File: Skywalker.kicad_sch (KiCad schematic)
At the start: 55 parts

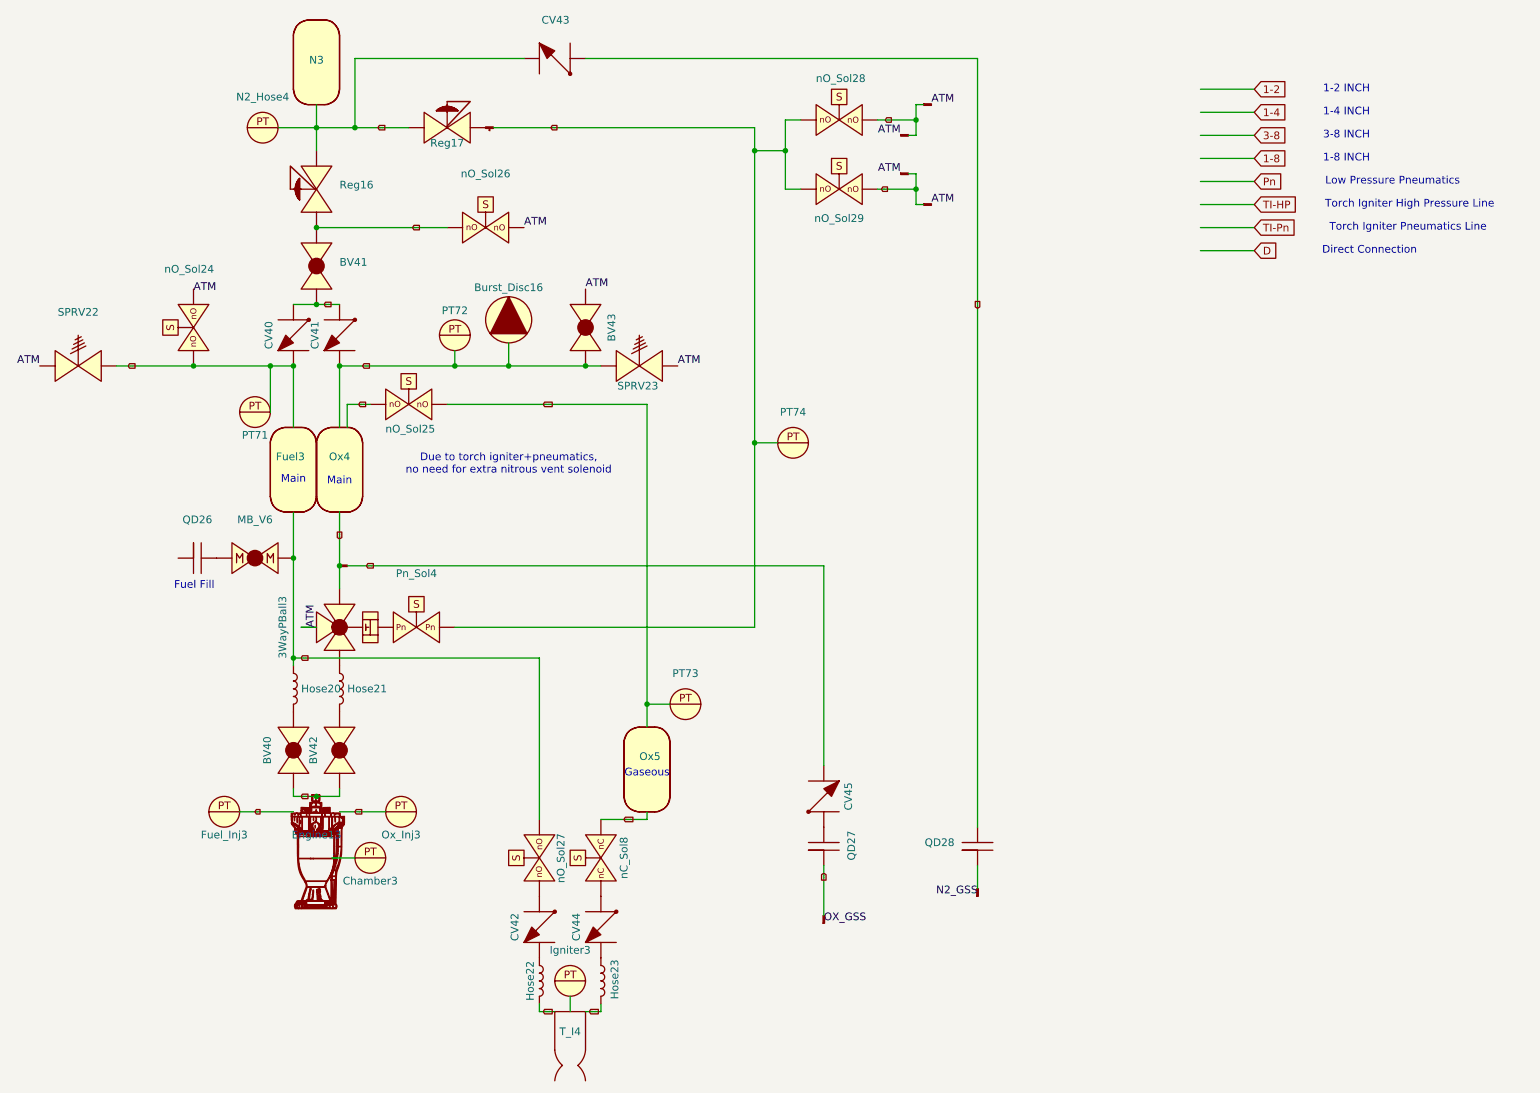
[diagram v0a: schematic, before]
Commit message: j0
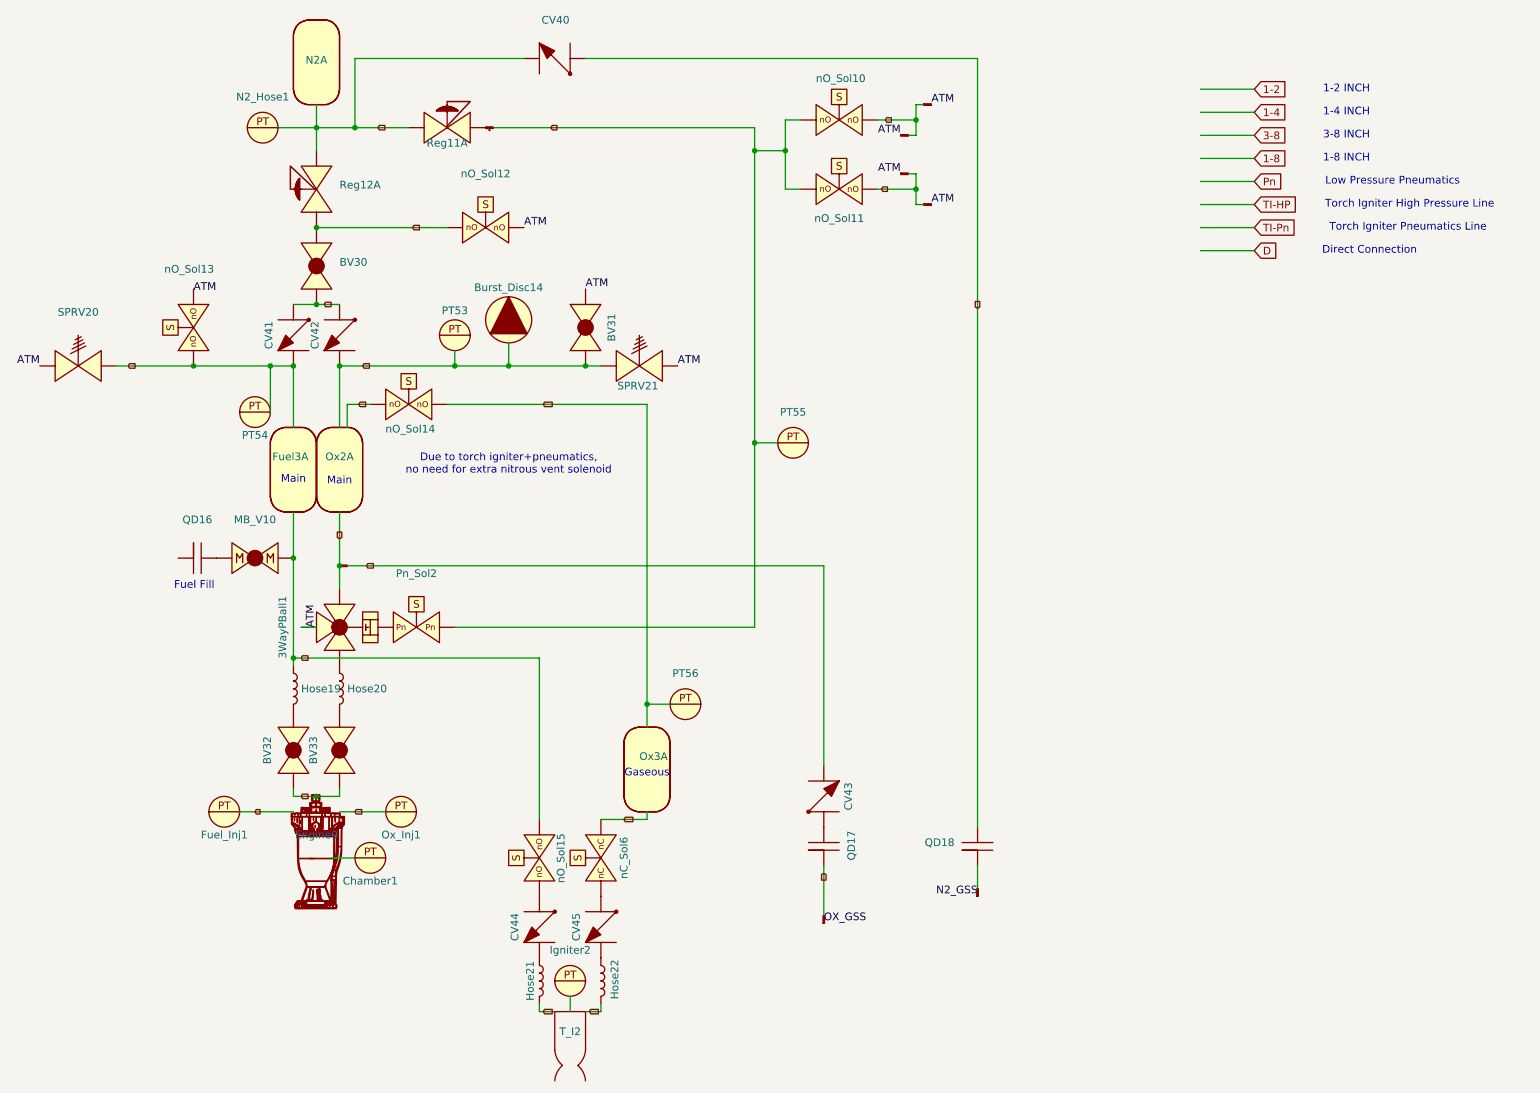
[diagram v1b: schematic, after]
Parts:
- renumbered 3WayPBall3 to 3WayPBall1, BV41 to BV30, BV43 to BV31, BV40 to BV32, BV42 to BV33, Burst_Disc16 to Burst_Disc14, CV43 to CV40, CV40 to CV41, CV41 to CV42, CV45 to CV43, CV42 to CV44, CV44 to CV45, Chamber3 to Chamber1, Engine13 to Engine9, Fuel_Inj3 to Fuel_Inj1, Hose20 to Hose19, Hose21 to Hose20, Hose22 to Hose21, Hose23 to Hose22, Igniter3 to Igniter2, MB_V6 to MB_V10, N3 to N2, N2_Hose4 to N2_Hose1, Ox4 to Ox2, Ox5 to Ox3, Ox_Inj3 to Ox_Inj1, PT72 to PT53, PT71 to PT54, PT74 to PT55, PT73 to PT56, Pn_Sol4 to Pn_Sol2, QD26 to QD16, QD27 to QD17, QD28 to QD18, Reg17 to Reg11, Reg16 to Reg12, SPRV22 to SPRV20, SPRV23 to SPRV21, Stop2 to Stop1, T_I4 to T_I2, U41 to U40, U39 to U41, U40 to U42, U42 to U43, U37 to U44, U43 to U45, U38 to U46, nC_Sol8 to nC_Sol6, nO_Sol28 to nO_Sol10, nO_Sol29 to nO_Sol11, nO_Sol26 to nO_Sol12, nO_Sol24 to nO_Sol13, nO_Sol25 to nO_Sol14, nO_Sol27 to nO_Sol15
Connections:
- net at CV45.: now also Hose22.1; no longer nC_Sol6.
- net at QD16.: now also MB_V10.
- new net: CV45., nC_Sol6.
- new net: Reg11., Stop1.
- new net: 3WayPBall1., Pn_Sol2.
- new net: CV43., QD17.
- new net: QD18., U45.

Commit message: more silwood stuff
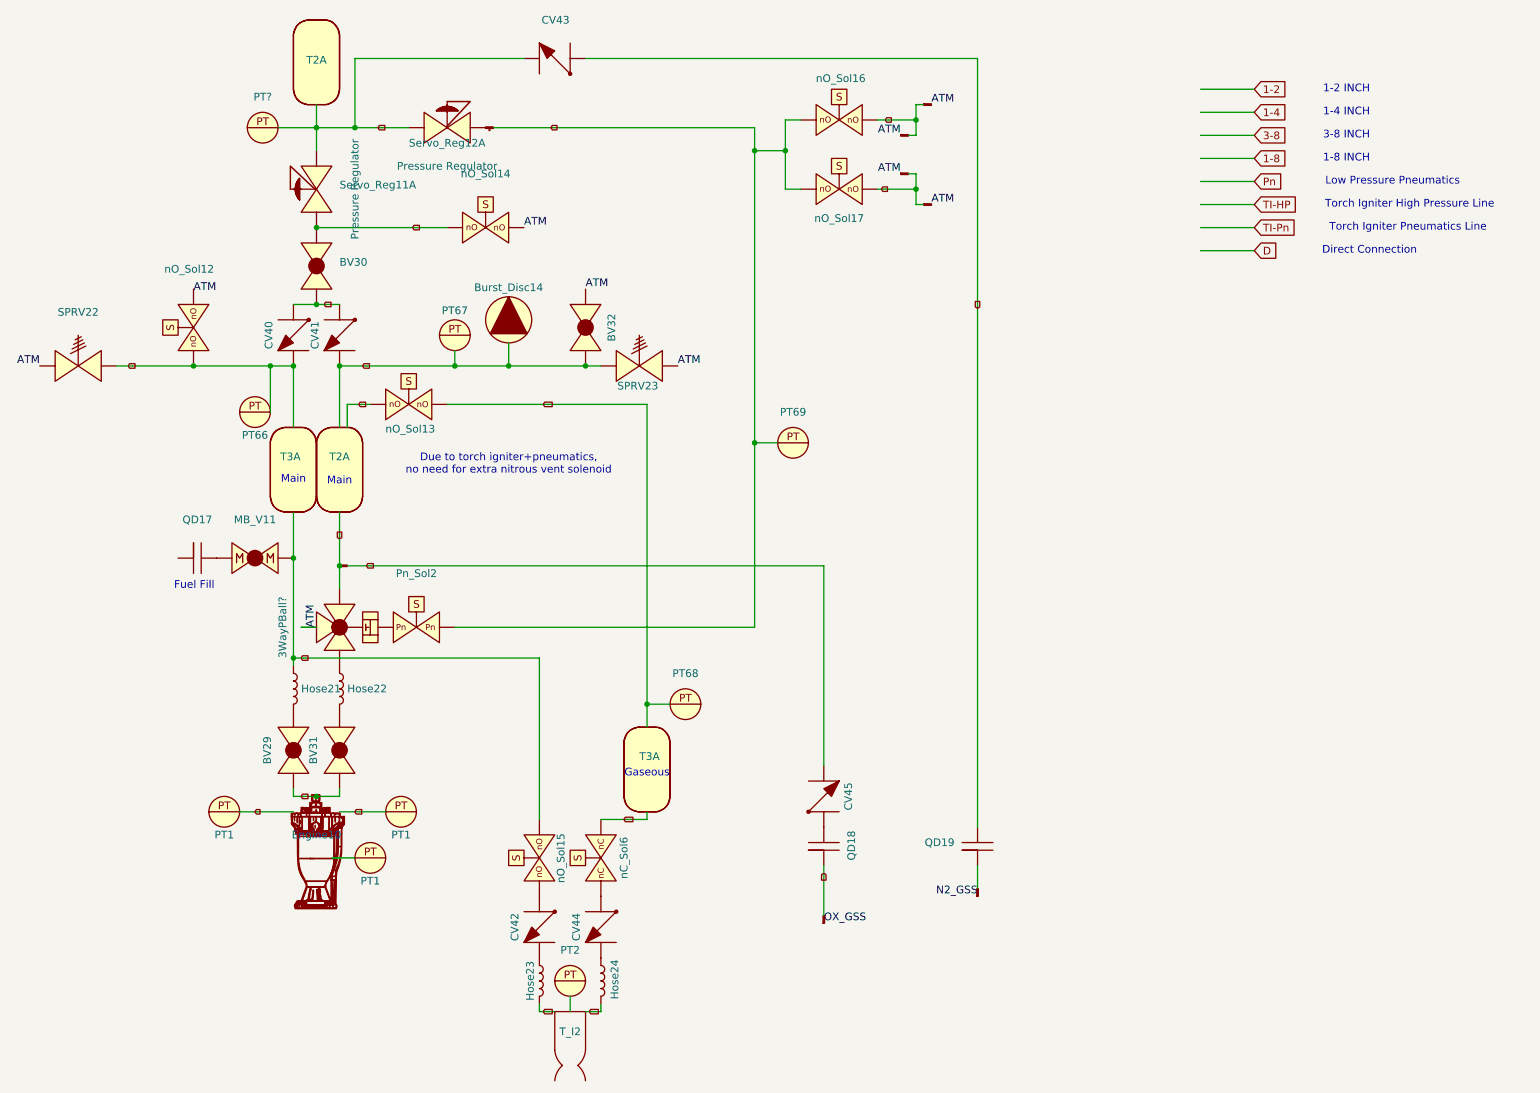
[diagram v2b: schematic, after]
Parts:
- renumbered 3WayPBall1 to 3WayPBall?, BV32 to BV29, BV33 to BV31, BV31 to BV32, CV41 to CV40, CV42 to CV41, CV44 to CV42, CV40 to CV43, CV45 to CV44, CV43 to CV45, Engine9 to Engine10, Hose19 to Hose21, Hose20 to Hose22, Hose21 to Hose23, Hose22 to Hose24, MB_V10 to MB_V11, Chamber1 to PT1, Fuel_Inj1 to PT1, Ox_Inj1 to PT1, Igniter2 to PT2, PT54 to PT66, PT53 to PT67, PT56 to PT68, PT55 to PT69, N2_Hose1 to PT?, QD16 to QD17, QD17 to QD18, QD18 to QD19, SPRV20 to SPRV22, SPRV21 to SPRV23, Reg12 to Servo_Reg11, Reg11 to Servo_Reg12, Ox2 to T2, N2 to T2, Fuel3 to T3, Ox3 to T3, U44 to U55, U46 to U56, U41 to U57, U42 to U58, U40 to U59, U43 to U60, U45 to U61, nO_Sol13 to nO_Sol12, nO_Sol14 to nO_Sol13, nO_Sol12 to nO_Sol14, nO_Sol10 to nO_Sol16, nO_Sol11 to nO_Sol17
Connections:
- net at CV44.: now also Hose24.1; no longer nC_Sol6.
- net at QD17.: now also MB_V11.
- new net: CV44., nC_Sol6.
- new net: Servo_Reg12., Stop1.
- new net: 3WayPBall?., Pn_Sol2.
- new net: CV45., QD18.
- new net: QD19., U61.

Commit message: Formatiing
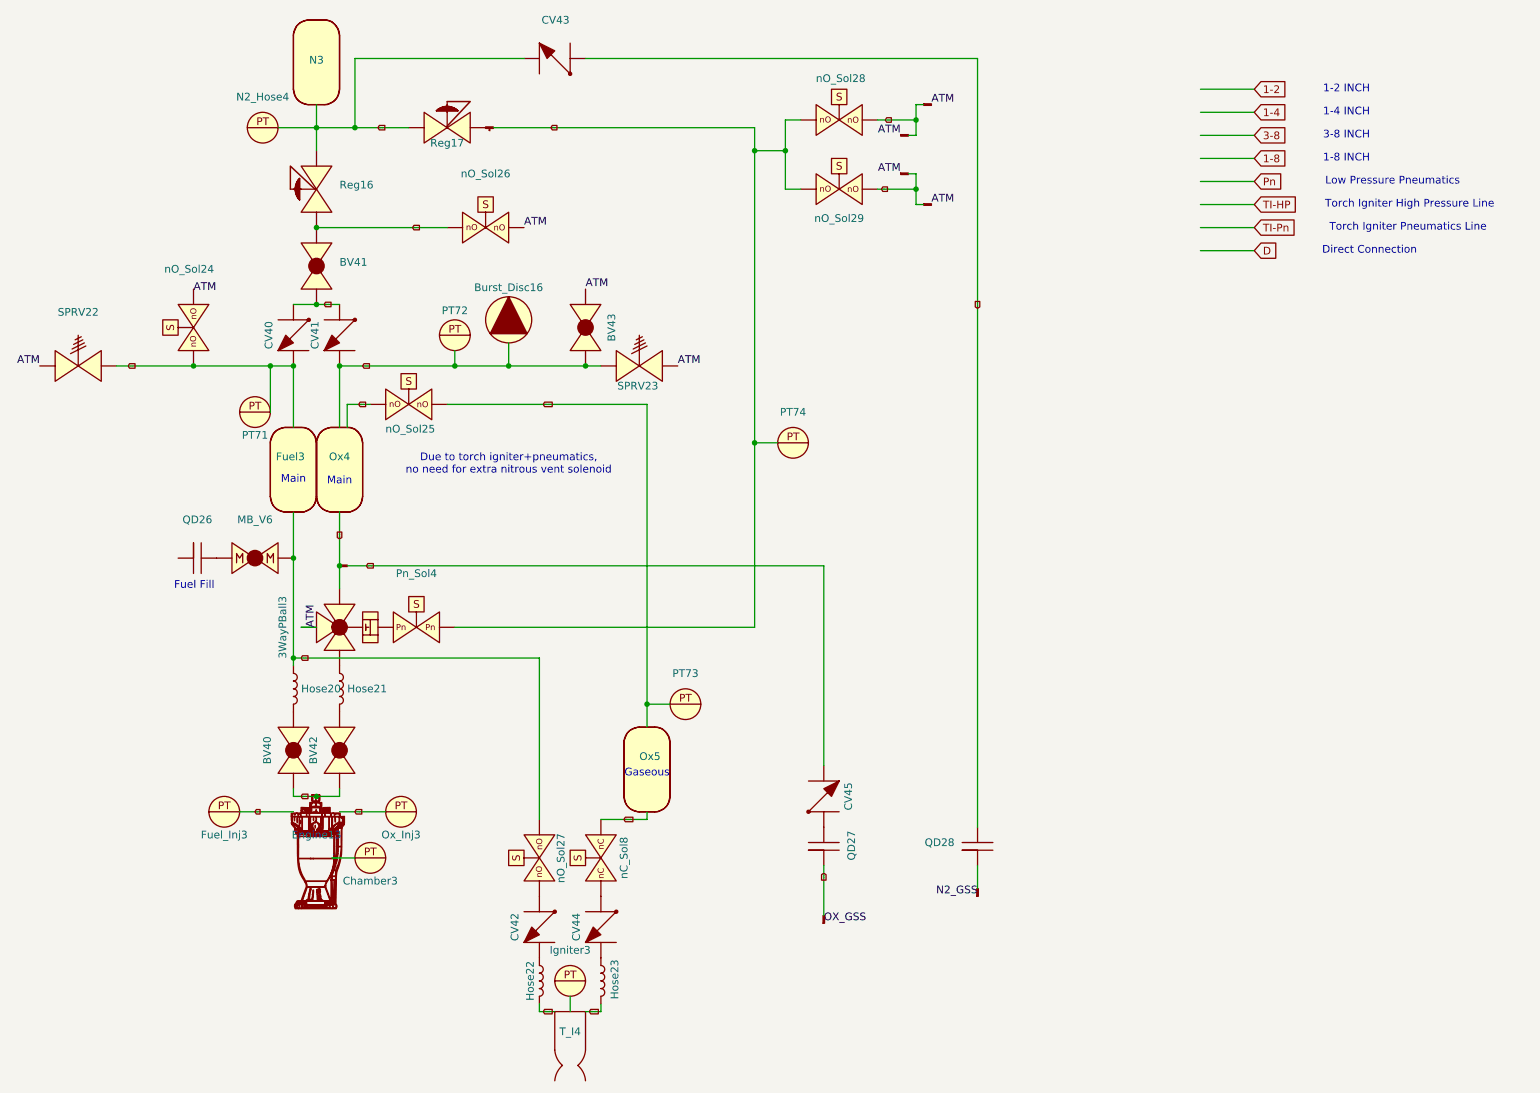
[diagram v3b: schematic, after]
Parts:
- gave numbers to parts that had none: 2
- renumbered BV29 to BV40, BV30 to BV41, BV31 to BV42, BV32 to BV43, Burst_Disc14 to Burst_Disc16, PT1 to Chamber3, Engine10 to Engine13, T3 to Fuel3, PT1 to Fuel_Inj3, Hose21 to Hose20, Hose22 to Hose21, Hose23 to Hose22, Hose24 to Hose23, PT2 to Igniter3, MB_V11 to MB_V6, T2 to N3, T2 to Ox4, T3 to Ox5, PT1 to Ox_Inj3, PT66 to PT71, PT67 to PT72, PT68 to PT73, PT69 to PT74, Pn_Sol2 to Pn_Sol4, QD17 to QD26, QD18 to QD27, QD19 to QD28, Servo_Reg11 to Reg16, Servo_Reg12 to Reg17, Stop1 to Stop2, T_I2 to T_I4, U55 to U37, U56 to U38, U57 to U39, U58 to U40, U59 to U41, U60 to U42, U61 to U43, nC_Sol6 to nC_Sol8, nO_Sol12 to nO_Sol24, nO_Sol13 to nO_Sol25, nO_Sol14 to nO_Sol26, nO_Sol15 to nO_Sol27, nO_Sol16 to nO_Sol28, nO_Sol17 to nO_Sol29
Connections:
- net at CV44.: now also Hose23.1; no longer nC_Sol8.
- net at QD26.: now also MB_V6.
- new net: CV44., nC_Sol8.
- new net: Reg17., Stop2.
- new net: 3WayPBall3., Pn_Sol4.
- new net: CV45., QD27.
- new net: QD28., U43.
